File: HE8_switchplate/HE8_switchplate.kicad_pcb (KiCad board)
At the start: 2 copper layers, 105.2 x 50 mm, 7 parts

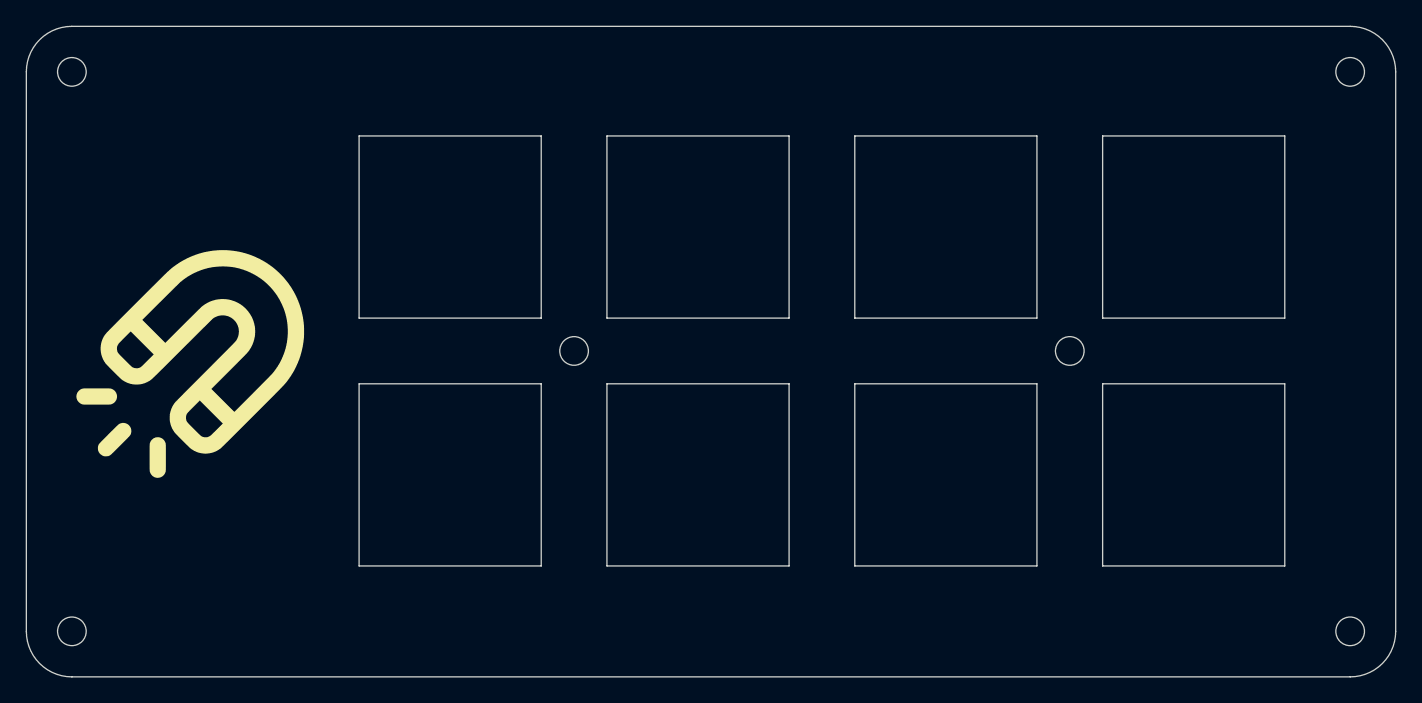
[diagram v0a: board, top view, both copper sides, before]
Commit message: add plate arts
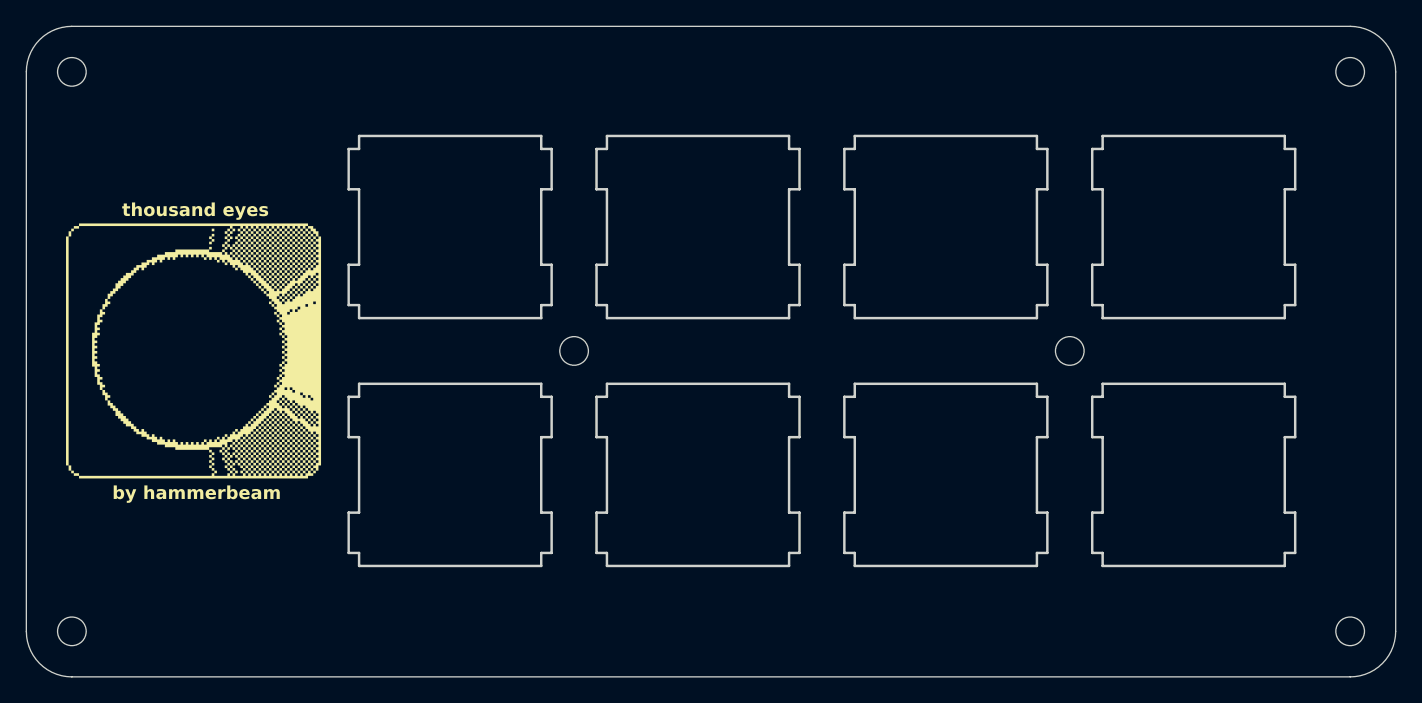
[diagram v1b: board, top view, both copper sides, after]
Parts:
- moved G*** 1.03 mm to (116.3, 78.2)
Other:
- outline, holes or cut-outs redrawn
- board text added: "by hammerbeam"
- board text added: "thousand eyes"
